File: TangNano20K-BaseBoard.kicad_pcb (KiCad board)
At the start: 2 copper layers, 100 x 85 mm, 49 parts, among them J1 Conn_01x20_Socket, J2 Conn_01x20_Socket, J3 Conn_01x06_Socket, J4 Conn_01x06_Socket, Q1 PN2222A, Q2 PN2222A, Q3 PN2222A, Q4 PN2222A, SW1 SW_SPDT_321, SW2 SW_SPDT_321, SW3 SW_SPDT_321, SW4 SW_SPDT_321, SW5 SW_SPDT_321, U1 CC56-12EWA, U2 SSD1306

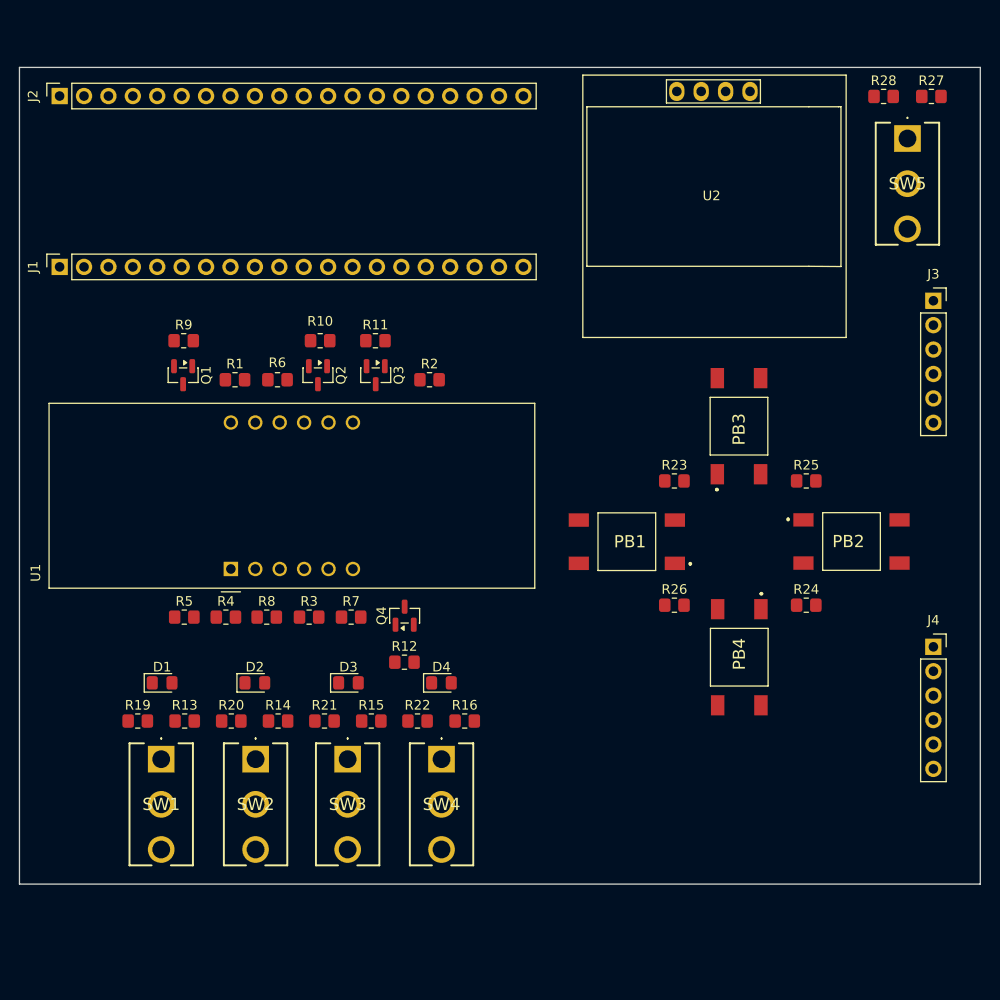
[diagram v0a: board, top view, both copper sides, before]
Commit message: Big Update
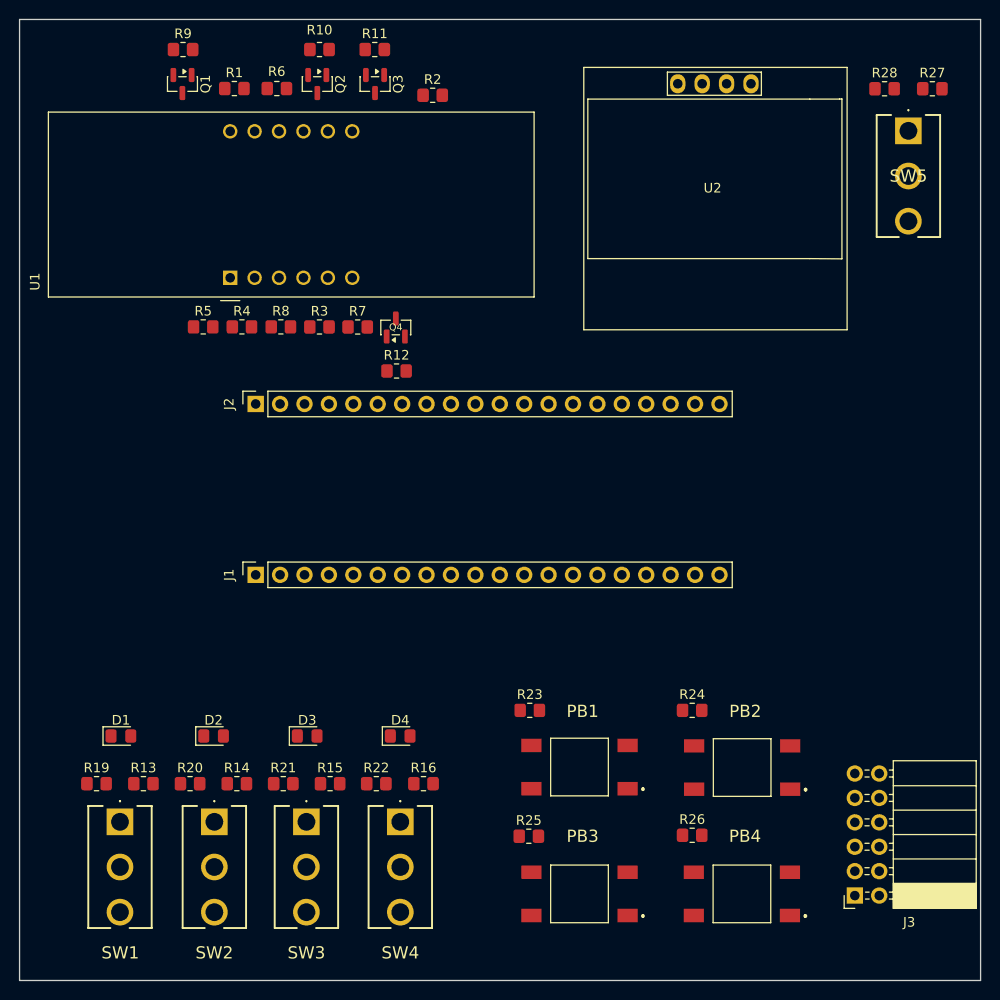
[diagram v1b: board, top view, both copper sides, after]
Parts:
- removed J4: Conn_01x06_Socket, Connector_PinSocket_2.54mm:PinSocket_1x06_P2.54mm_Vertical
- J3: value Conn_01x06_Socket -> Conn_02x06_Odd_Even; footprint Connector_PinSocket_2.54mm:PinSocket_1x06_P2.54mm_Vertical -> Connector_PinSocket_2.54mm:PinSocket_2x06_P2.54mm_Horizontal
- moved J3 62.4 mm to (236.9, 161.2), turned to 180 degrees
- moved PB3 50.3 mm to (209.1, 161.0), turned to 180 degrees
- moved R25 46.9 mm to (203.0, 155.0)
- moved J1 38.0 mm to (174.6, 127.8)
- moved J2 38.0 mm to (174.6, 110.0)
- moved R12 30.3 mm to (189.2, 106.6)
- moved Q1 30.3 mm to (167.0, 76.7)
- moved Q2 30.3 mm to (181.0, 76.7)
- moved Q3 30.3 mm to (187.0, 76.7)
- moved R1 30.3 mm to (172.4, 77.2)
- moved R10 30.3 mm to (181.2, 73.1)
- moved R11 30.3 mm to (187.0, 73.1)
- moved R6 30.3 mm to (176.8, 77.2)
- moved R9 30.3 mm to (167.0, 73.1)
- moved U1 30.3 mm to (171.9, 96.9)
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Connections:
- J3 pad 1: /80 -> +3V3
- J3 pad 2: /41 -> +3V3
- J3 pad 3: /55 -> GND
- J3 pad 4: /49 -> GND
- J3 pad 5: +3V3 -> /80
- J3 pad 6: GND -> /86
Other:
- board size 100 x 85 mm -> 100 x 100 mm
- board text added: "Q4"
